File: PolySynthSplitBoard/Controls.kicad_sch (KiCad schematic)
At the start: 105 parts, among them SW601 ENV1_B, SW602 ENV2_B, SW603 HP_B, SW604 LFO1_B, SW605 LFO2_B, SW606 HP_B, SW607 LFO3_B, SW608 FF_B, SW609 MIX1_B, SW610 MIX2_B, SW611 ENC_MENU, SW612 ALT_B, U601 MCP23S17_SS, U602 MCP23S17_SS, U603 ILI9341

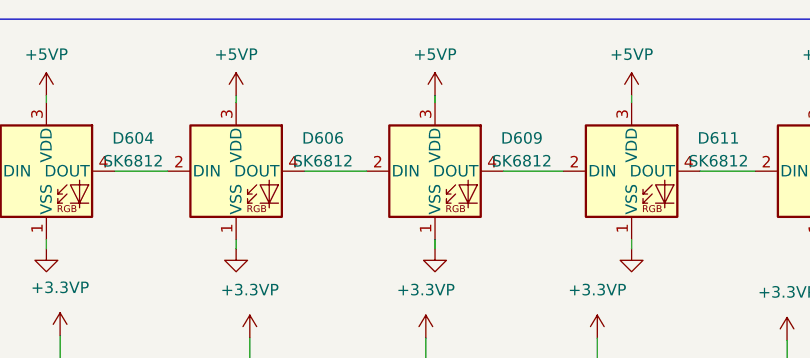
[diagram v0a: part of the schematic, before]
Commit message: rev2 motherboard sent to fab
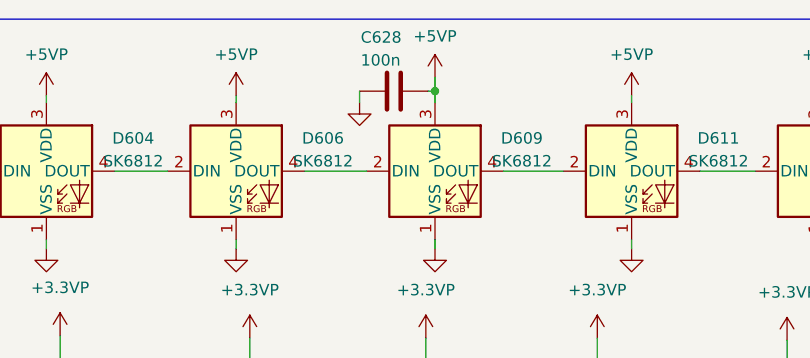
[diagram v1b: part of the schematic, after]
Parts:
- added C628: 100n, Capacitor_SMD:C_0805_2012Metric, symbol Device:C
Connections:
- net +5VP: now also C628.2
- net GNDA: now also C628.1
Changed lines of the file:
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@@
 	)
 	(junction
+		(at 109.22 24.384)
+		(diameter 0)
+		(color 0 0 0 0)
+	)
+	(junction
 		(at 266.192 80.772)
 		(diameter 0)
@@
 	(wire
 		(pts
+			(xy 109.22 24.384) (xy 109.22 25.654)
+		)
+		(stroke
+			(width 0)
+			(type default)
+		)
+	)
+	(wire
+		(pts
 			(xy 251.714 181.356) (xy 254.762 181.356)
 		)
@@
 	(wire
 		(pts
-			(xy 109.22 24.892) (xy 109.22 25.654)
+			(xy 109.22 22.86) (xy 109.22 24.384)
 		)
 		(stroke
@@
 	(wire
 		(pts
+			(xy 100.838 24.384) (xy 100.838 25.654)
+		)
+		(stroke
+			(width 0)
+			(type default)
+		)
+	)
+	(wire
+		(pts
 			(xy 51.308 207.264) (xy 51.308 199.898)
 		)
@@
 	(wire
 		(pts
+			(xy 108.458 24.384) (xy 109.22 24.384)
+		)
+		(stroke
+			(width 0)
+			(type default)
+		)
+	)
+	(wire
+		(pts
 			(xy 73.66 33.274) (xy 79.502 33.274)
 		)
@@
 	)
 	(symbol
+		(lib_id "Device:C")
+		(at 104.648 24.384 90)
+		(unit 1)
+		(exclude_from_sim no)
+		(in_bom yes)
+		(on_board yes)
+		(dnp no)
+		(property "Reference" "C628"
+			(at 100.965 18.415 90)
+			(effects
+				(font
+					(size 1.27 1.27)
+				)
+				(justify right)
+			)
+		)
+		(property "Value" "100n"
+			(at 100.965 20.955 90)
+			(effects
+				(font
+					(size 1.27 1.27)
+				)
+				(justify right)
+			)
+		)
+		(property "Footprint" "Capacitor_SMD:C_0805_2012Metric"
+			(at 108.458 23.4188 0)
+			(effects
+				(font
+					(size 1.27 1.27)
+				)
+				(hide yes)
+			)
+		)
+		(property "Datasheet" "~"
+			(at 104.648 24.384 0)
+			(effects
+				(font
+					(size 1.27 1.27)
+				)
+				(hide yes)
+			)
+		)
+		(property "Description" ""
+			(at 104.648 24.384 0)
+			(effects
+				(font
+					(size 1.27 1.27)
+				)
+				(hide yes)
+			)
+		)
+		(pin "1"
+		)
+		(pin "2"
+		)
+		(instances
+			(project "PolySynthSplitBoard"
+				(path "/22649217-9810-470f-bc7b-6f743ad2b90e/db382c1e-7a8e-4aae-96bd-96ec756a5476/f9611335-018a-4682-8f39-2088bfa85de9"
+					(reference "C628")
+					(unit 1)
+				)
+			)
+		)
+	)
+	(symbol
 		(lib_id "Device:R_US")
 		(at 88.646 58.928 0)
@@
 	)
 	(symbol
+		(lib_id "power:GND")
+		(at 100.838 25.654 0)
+		(unit 1)
+		(exclude_from_sim no)
+		(in_bom yes)
+		(on_board yes)
+		(dnp no)
+		(fields_autoplaced yes)
+		(property "Reference" "#PWR0870"
+			(at 100.838 32.004 0)
+			(effects
+				(font
+					(size 1.27 1.27)
+				)
+				(hide yes)
+			)
+		)
+		(property "Value" "GNDA"
+			(at 100.838 29.464 0)
+			(effects
+				(font
+					(size 1.27 1.27)
+				)
+				(hide yes)
+			)
+		)
+		(property "Footprint" ""
+			(at 100.838 25.654 0)
+			(effects
+				(font
+					(size 1.27 1.27)
+				)
+				(hide yes)
+			)
+		)
+		(property "Datasheet" ""
+			(at 100.838 25.654 0)
+			(effects
+				(font
+					(size 1.27 1.27)
+				)
+				(hide yes)
+			)
+		)
+		(property "Description" ""
+			(at 100.838 25.654 0)
+			(effects
+				(font
+					(size 1.27 1.27)
+				)
+				(hide yes)
+			)
+		)
+		(pin "1"
+		)
+		(instances
+			(project "PolySynthSplitBoard"
+				(path "/22649217-9810-470f-bc7b-6f743ad2b90e/db382c1e-7a8e-4aae-96bd-96ec756a5476/f9611335-018a-4682-8f39-2088bfa85de9"
+					(reference "#PWR0870")
+					(unit 1)
+				)
+			)
+		)
+	)
+	(symbol
 		(lib_id "Device:C")
 		(at 109.474 112.268 0)
@@
 	(symbol
 		(lib_id "power:+5VP")
-		(at 109.22 24.892 0)
+		(at 109.22 22.86 0)
 		(unit 1)
 		(exclude_from_sim no)
@@
 		(fields_autoplaced yes)
 		(property "Reference" "#PWR0697"
-			(at 109.22 28.702 0)
+			(at 109.22 26.67 0)
 			(effects
 				(font
@@
 		)
 		(property "Value" "+5VP"
-			(at 109.22 20.32 0)
+			(at 109.22 18.288 0)
 			(effects
 				(font
@@
 		)
 		(property "Footprint" ""
-			(at 109.22 24.892 0)
+			(at 109.22 22.86 0)
 			(effects
 				(font
@@
 		)
 		(property "Datasheet" ""
-			(at 109.22 24.892 0)
+			(at 109.22 22.86 0)
 			(effects
 				(font
@@
 		)
 		(property "Description" "Power symbol creates a global label with name \"+5VP\""
-			(at 109.22 24.892 0)
+			(at 109.22 22.86 0)
 			(effects
 				(font
